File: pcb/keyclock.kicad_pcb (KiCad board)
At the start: 2 copper layers, 11 parts, among them J1 Conn_01x08_Pin, SW1 SW_Push, SW2 SW_Push, SW3 SW_Push, SW4 SW_Push, U1 XIAO-ESP32-C3-SMD

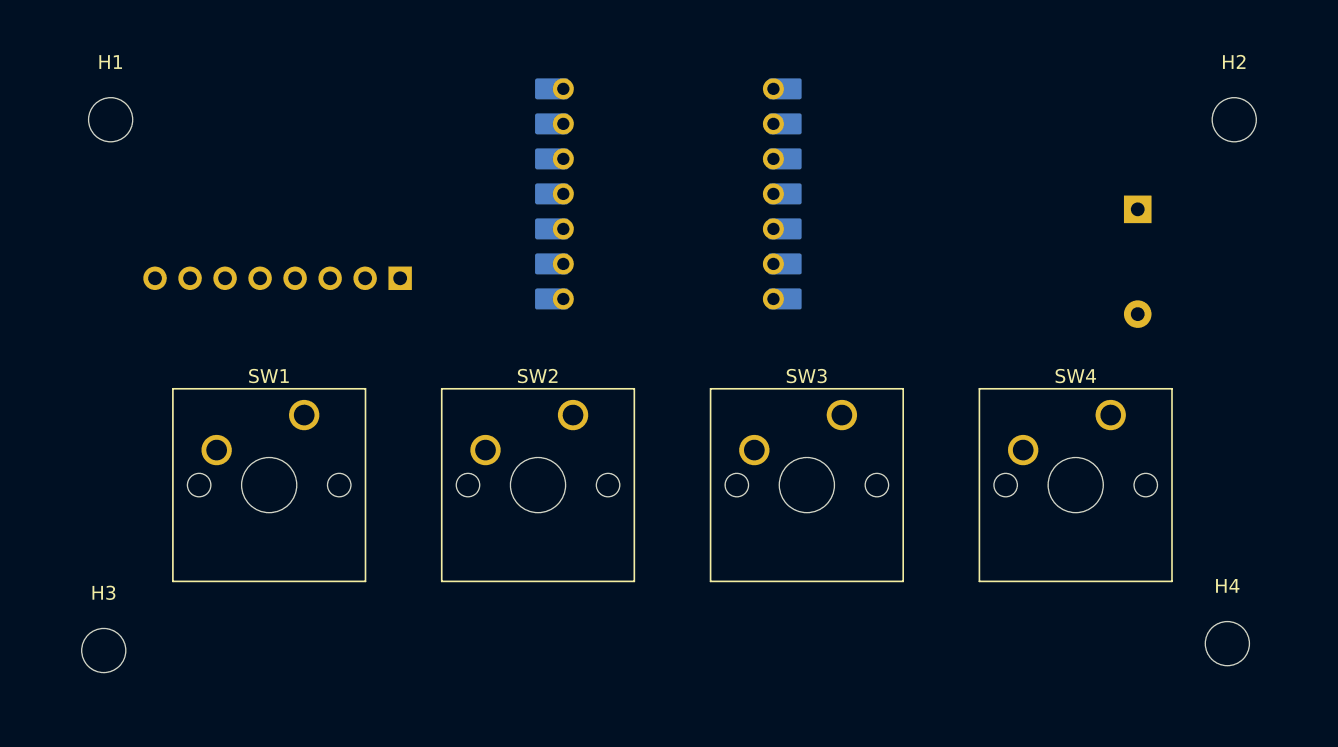
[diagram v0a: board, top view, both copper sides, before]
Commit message: Finish PCB routing and design
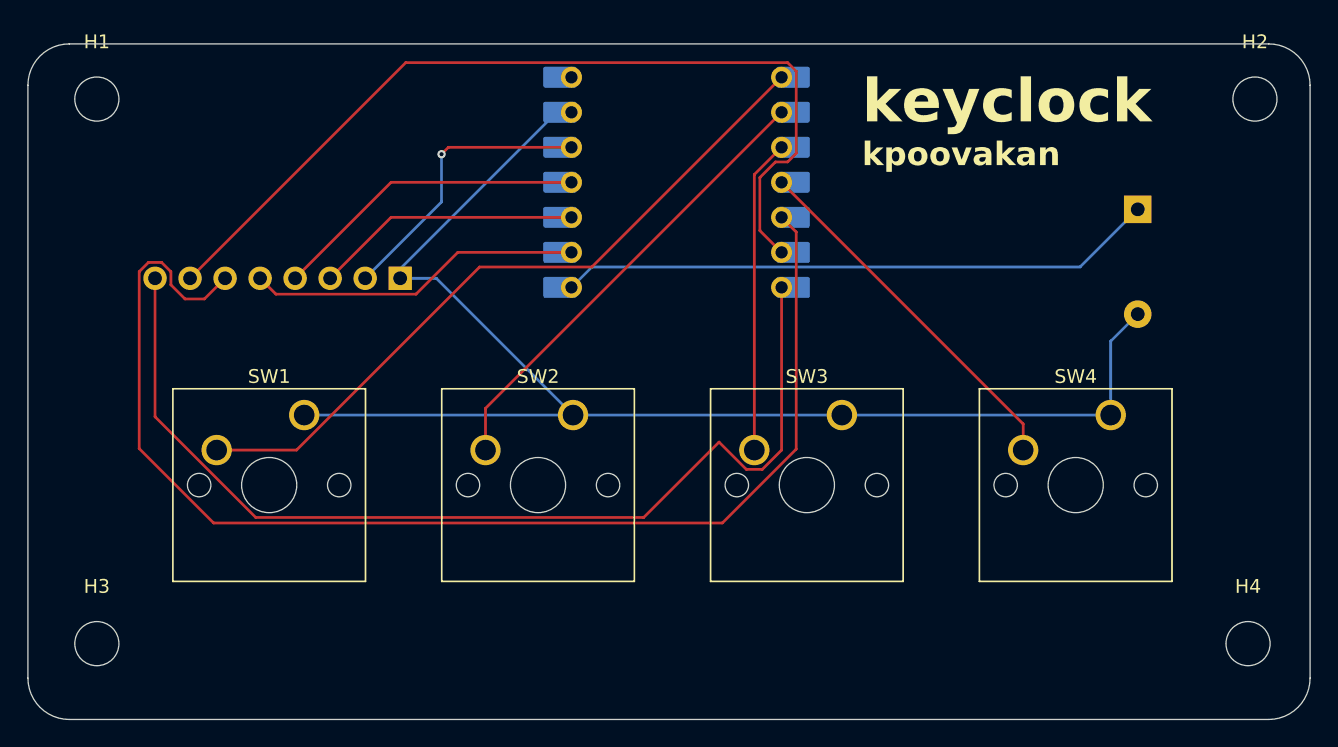
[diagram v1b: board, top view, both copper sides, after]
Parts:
- moved H2 2.12 mm to (186.0, 110.0)
- moved H1 1.80 mm to (102.0, 110.0)
- moved H4 1.50 mm to (185.5, 149.5)
- moved U1 1.03 mm to (144.0, 116.0)
- moved H3 0.71 mm to (102.0, 149.5)
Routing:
- net GND: track 0.00 -> 101.1 mm
- net /DC: track 0.00 -> 91.0 mm
- net /BL: track 0.00 -> 74.0 mm
- net /CS: track 0.00 -> 66.1 mm
- net Net-(U1-D0): track 0.00 -> 52.2 mm
- net Net-(BZ1-+): track 0.00 -> 43.4 mm
- net Net-(U1-D1): track 0.00 -> 33.4 mm
- net Net-(U1-D3): track 0.00 -> 26.7 mm
- net /RST: track 0.00 -> 24.3 mm
- net /SDA: track 0.00 -> 22.9 mm
- net Net-(U1-D2): track 0.00 -> 22.8 mm
- net +3V3: track 0.00 -> 20.9 mm, vias 0 -> 1
- net /SCL: track 0.00 -> 19.3 mm
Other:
- board outline added: 93 x 49 mm
- board text added: "keyclock"
- board text added: "kpoovakan"
